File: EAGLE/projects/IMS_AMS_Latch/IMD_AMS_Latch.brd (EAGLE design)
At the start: 55.9 x 65.7 mm, 17 parts, among them CON1 T821108A1S100CEU, CON2 T821108A1S100CEU, IC1 4011N, K1 EC2-12TNU, K2 EC2-12TNU, T1 BT169, T2 BT169

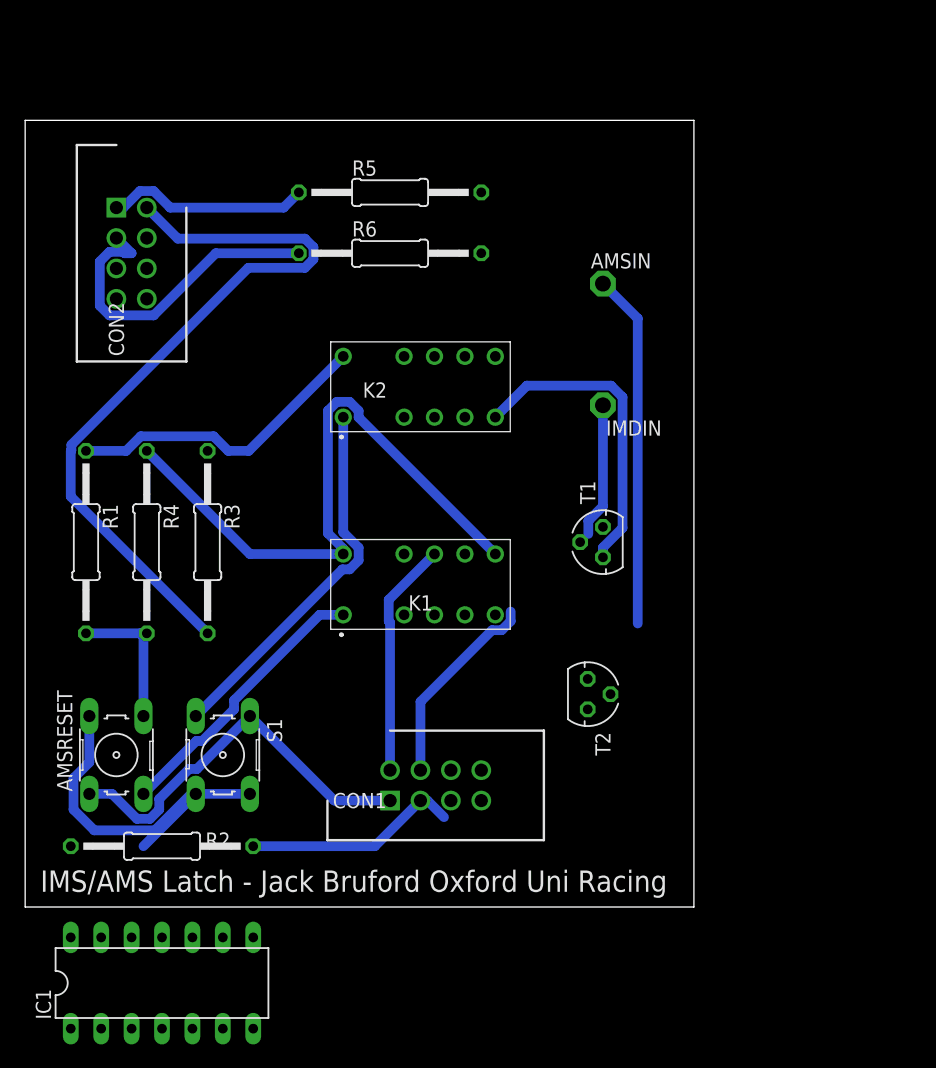
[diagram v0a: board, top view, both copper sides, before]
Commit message: Update for workshop
Signed-off-by: Jack Bruford <jack.bruford41@gmail.com>
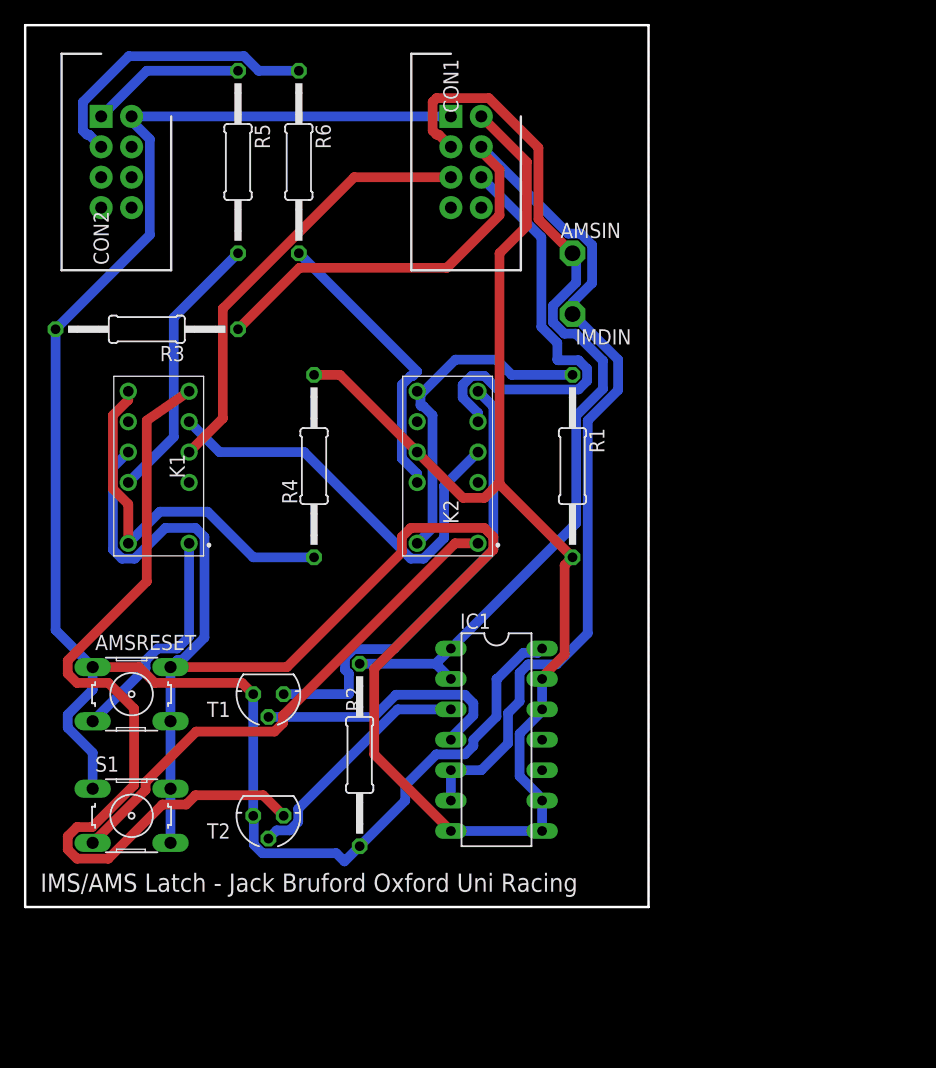
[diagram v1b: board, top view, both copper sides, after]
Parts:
- moved CON1 57.4 mm to (35.6, 66.0), turned to 270 degrees
- moved R1 41.1 mm to (45.7, 36.8)
- moved IC1 34.5 mm to (39.4, 14.0), turned to 270 degrees
- moved T1 30.7 mm to (20.3, 17.8), turned to 180 degrees
- moved T2 28.5 mm to (20.3, 7.62), turned to 180 degrees
- moved K1 23.9 mm to (11.4, 36.8), turned to 90 degrees
- moved R3 18.5 mm to (10.2, 48.3), turned to 180 degrees
- moved R2 18.2 mm to (27.9, 12.7), turned to 270 degrees
- moved R4 15.3 mm to (24.1, 36.8), turned to 90 degrees
- moved R5 13.0 mm to (17.8, 62.2), turned to 270 degrees
- moved R6 10.8 mm to (22.9, 62.2), turned to 270 degrees
- moved S1 9.16 mm to (8.89, 7.62), turned to 0 degrees
- moved IMDIN 8.03 mm to (45.7, 49.5)
- moved CON2 7.73 mm to (6.35, 66.0)
- moved K2 6.84 mm to (35.6, 36.8), turned to 90 degrees
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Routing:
- net GND: track 62.9 -> 204.3 mm
- net IMDIN: track 28.1 -> 102.1 mm
- net N$2: track 0.00 -> 71.0 mm
- net +12V: track 96.4 -> 151.6 mm
- net ESDC+: track 0.00 -> 36.8 mm
- net ESDC-: track 0.00 -> 36.7 mm
- net IMSRESET: track 0.00 -> 35.1 mm
- net AMSIN: track 47.7 -> 76.6 mm
- net N$7: track 0.00 -> 24.4 mm
- net AMSLED: track 0.00 -> 22.9 mm
- net N$11: track 0.00 -> 22.0 mm
- net N$6: track 52.3 -> 31.9 mm
- net N$10: track 0.00 -> 20.3 mm
- net N$4: track 26.2 -> 38.5 mm
- net N$5: track 31.5 -> 43.3 mm
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- added copper zone on layer 1, net GND
- added copper zone on layer 16, net GND
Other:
- board size 55.9 x 65.7 mm -> 52.1 x 73.7 mm
